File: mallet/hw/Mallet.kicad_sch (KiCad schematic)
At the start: 24 parts, among them J1 Conn_01x05, J2 Conn_01x03, J3 Conn_01x04, J4 Conn_01x04, U1 STM32G030F6Px, U2 AS5600L-ASOM, U3 DRV8313PWPR

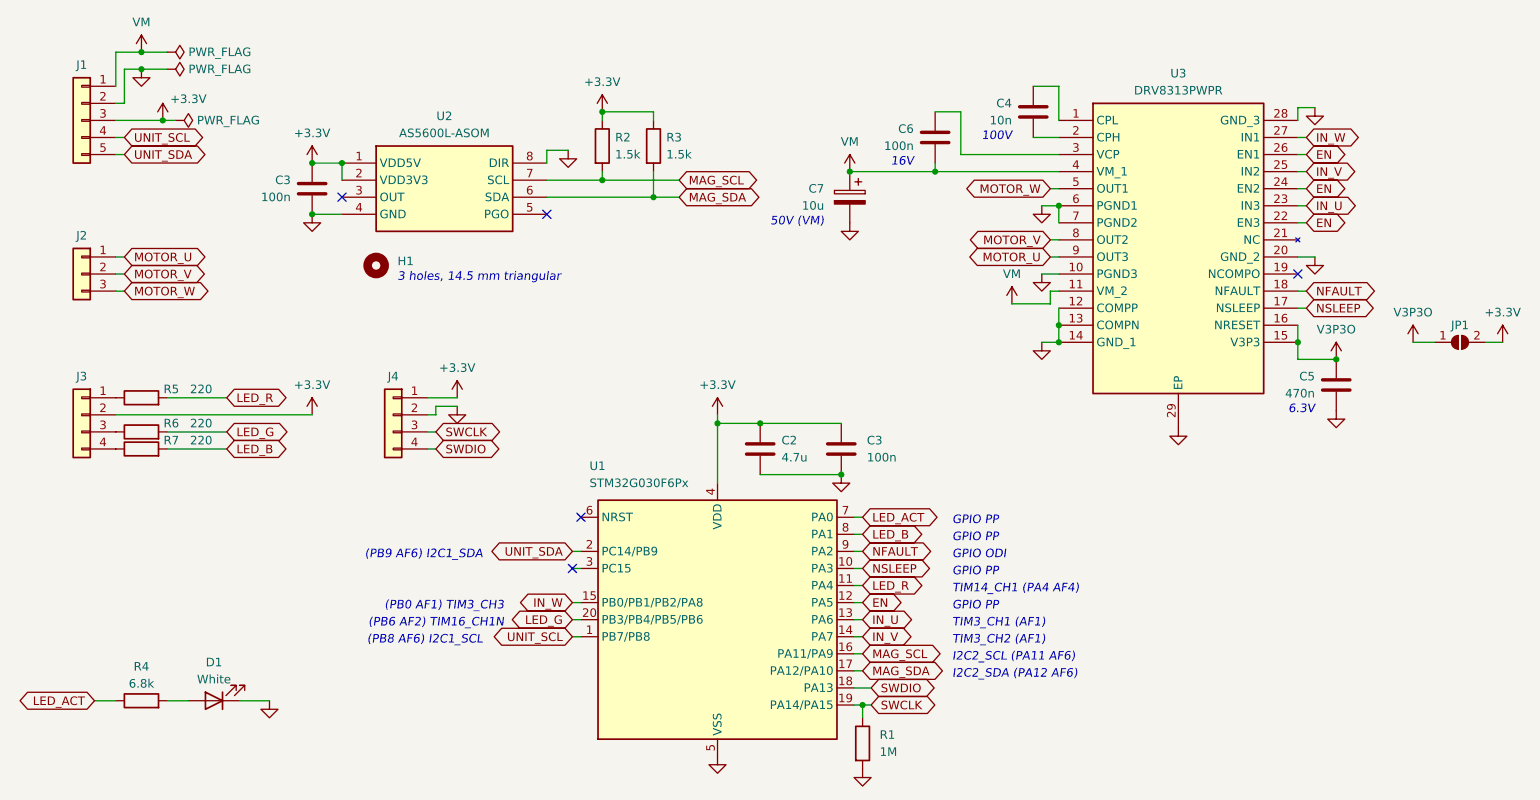
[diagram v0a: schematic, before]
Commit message: Finish mallet PCB
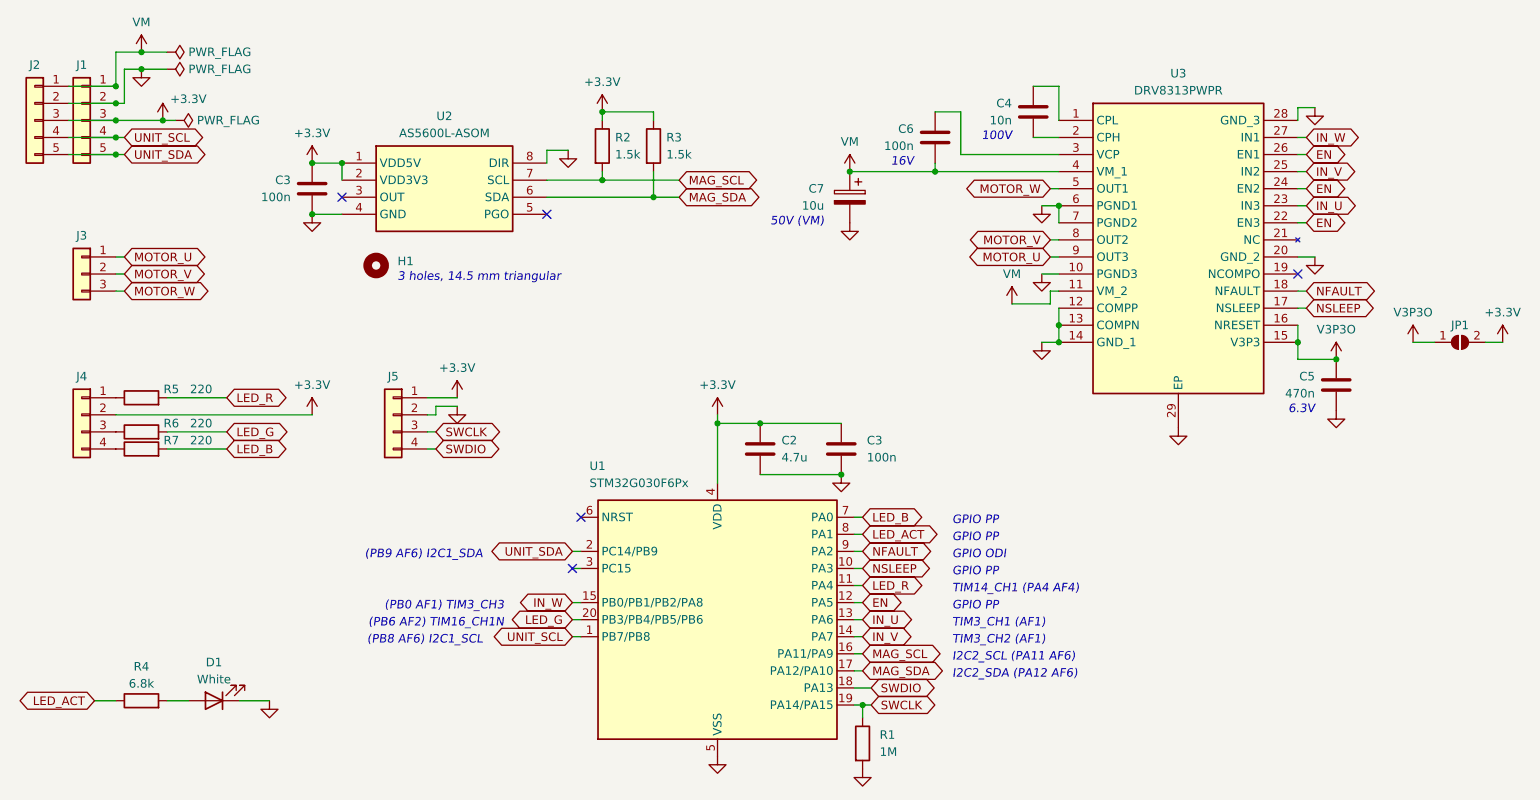
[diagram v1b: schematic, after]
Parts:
- added J2: Conn_01x05, Connector_PinHeader_2.00mm:PinHeader_1x05_P2.00mm_Vertical, symbol Connector_Generic:Conn_01x05
- C5: footprint Capacitor_SMD:C_0805_2012Metric -> Capacitor_SMD:C_0603_1608Metric
- J1: footprint Connector_PinHeader_2.00mm:PinHeader_1x04_P2.00mm_Vertical -> Connector_PinHeader_2.00mm:PinHeader_1x05_P2.00mm_Vertical
- renumbered J2 to J3, J3 to J4, J4 to J5
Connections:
- net +3.3V: now also J2.3 (Pin_3)
- net GND: now also J2.2 (Pin_2)
- net LED_ACT: now also U1.8 (PA1); no longer U1.7 (PA0)
- net LED_B: now also U1.7 (PA0); no longer U1.8 (PA1)
- net UNIT_SCL: now also J2.4 (Pin_4)
- net UNIT_SDA: now also J2.5 (Pin_5)
- net VM: now also J2.1 (Pin_1)
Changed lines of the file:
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@@
   (junction (at 156.845 38.735) (diameter 0) (color 0 0 0 0)
   )
+  (junction (at 34.925 26.035) (diameter 0) (color 0 0 0 0)
+  )
   (junction (at 175.26 61.595) (diameter 0) (color 0 0 0 0)
   )
@@
   (junction (at 114.935 42.545) (diameter 0) (color 0 0 0 0)
   )
+  (junction (at 34.925 31.115) (diameter 0) (color 0 0 0 0)
+  )
+  (junction (at 34.925 28.575) (diameter 0) (color 0 0 0 0)
+  )
   (junction (at 175.26 64.135) (diameter 0) (color 0 0 0 0)
   )
   (junction (at 38.735 20.955) (diameter 0) (color 0 0 0 0)
   )
+  (junction (at 34.925 33.655) (diameter 0) (color 0 0 0 0)
+  )
   (junction (at 68.58 37.465) (diameter 0) (color 0 0 0 0)
+  )
+  (junction (at 34.925 36.195) (diameter 0) (color 0 0 0 0)
   )
   (junction (at 124.46 76.2) (diameter 0) (color 0 0 0 0)
@@
     (stroke (width 0) (type default))
   )
+  (wire (pts (xy 27.94 33.655) (xy 34.925 33.655))
+    (stroke (width 0) (type default))
+  )
   (wire (pts (xy 146.05 92.71) (xy 144.78 92.71))
     (stroke (width 0) (type default))
@@
     (stroke (width 0) (type default))
   )
+  (wire (pts (xy 27.94 31.115) (xy 34.925 31.115))
+    (stroke (width 0) (type default))
+  )
   (wire (pts (xy 114.935 42.545) (xy 99.06 42.545))
     (stroke (width 0) (type default))
   )
+  (wire (pts (xy 27.94 28.575) (xy 34.925 28.575))
+    (stroke (width 0) (type default))
+  )
   (wire (pts (xy 227.965 64.135) (xy 231.14 64.135))
     (stroke (width 0) (type default))
@@
     (stroke (width 0) (type default))
   )
+  (wire (pts (xy 27.94 26.035) (xy 34.925 26.035))
+    (stroke (width 0) (type default))
+  )
   (wire (pts (xy 147.32 118.11) (xy 146.05 118.11))
     (stroke (width 0) (type default))
   )
   (wire (pts (xy 212.09 43.815) (xy 210.82 43.815))
+    (stroke (width 0) (type default))
+  )
+  (wire (pts (xy 27.94 36.195) (xy 34.925 36.195))
     (stroke (width 0) (type default))
   )
@@
     )
   )
-  (global_label "LED_B" (shape bidirectional) (at 146.05 92.71 0) (fields_autoplaced)
-    (effects (font (size 1.27 1.27)) (justify left))
-    (property "Intersheetrefs" "${INTERSHEET_REFS}" (at 155.8312 92.71 0)
+  (global_label "LED_ACT" (shape bidirectional) (at 146.05 92.71 0) (fields_autoplaced)
+    (effects (font (size 1.27 1.27)) (justify left))
+    (property "Intersheetrefs" "${INTERSHEET_REFS}" (at 157.8874 92.71 0)
       (effects (font (size 1.27 1.27)) (justify left) hide)
     )
@@
     )
   )
-  (global_label "LED_ACT" (shape bidirectional) (at 146.05 90.17 0) (fields_autoplaced)
-    (effects (font (size 1.27 1.27)) (justify left))
-    (property "Intersheetrefs" "${INTERSHEET_REFS}" (at 157.8874 90.17 0)
+  (global_label "LED_B" (shape bidirectional) (at 146.05 90.17 0) (fields_autoplaced)
+    (effects (font (size 1.27 1.27)) (justify left))
+    (property "Intersheetrefs" "${INTERSHEET_REFS}" (at 155.8312 90.17 0)
       (effects (font (size 1.27 1.27)) (justify left) hide)
     )
@@
       (effects (font (size 1.27 1.27)) (justify left))
     )
-    (property "Footprint" "Capacitor_SMD:C_0805_2012Metric" (at 215.5698 74.295 0)
+    (property "Footprint" "Capacitor_SMD:C_0603_1608Metric" (at 215.5698 74.295 0)
       (effects (font (size 1.27 1.27)) hide)
     )
@@
   (symbol (lib_id "Connector_Generic:Conn_01x03") (at 29.845 53.975 0) (mirror y) (unit 1)
     (in_bom yes) (on_board yes) (dnp no)
-    (property "Reference" "J2" (at 29.845 48.26 0)
+    (property "Reference" "J3" (at 29.845 48.26 0)
       (effects (font (size 1.27 1.27)))
     )
@@
       (project "Mallet"
         (path "/503c6fae-2261-4b98-b430-844cd1712448"
-          (reference "J2") (unit 1)
+          (reference "J3") (unit 1)
         )
       )
@@
   (symbol (lib_id "Connector_Generic:Conn_01x04") (at 76.2 74.93 0) (mirror y) (unit 1)
     (in_bom yes) (on_board yes) (dnp no)
-    (property "Reference" "J4" (at 76.2 69.215 0)
+    (property "Reference" "J5" (at 76.2 69.215 0)
       (effects (font (size 1.27 1.27)))
     )
@@
       (project "Mallet"
         (path "/503c6fae-2261-4b98-b430-844cd1712448"
-          (reference "J4") (unit 1)
+          (reference "J5") (unit 1)
         )
       )
@@
   (symbol (lib_id "Connector_Generic:Conn_01x04") (at 29.845 74.93 0) (mirror y) (unit 1)
     (in_bom yes) (on_board yes) (dnp no)
-    (property "Reference" "J3" (at 29.845 69.215 0)
+    (property "Reference" "J4" (at 29.845 69.215 0)
       (effects (font (size 1.27 1.27)))
     )
@@
       (project "Mallet"
         (path "/503c6fae-2261-4b98-b430-844cd1712448"
-          (reference "J3") (unit 1)
+          (reference "J4") (unit 1)
         )
       )
@@
       (effects (font (size 1.27 1.27)) hide)
     )
-    (property "Footprint" "Connector_PinHeader_2.00mm:PinHeader_1x04_P2.00mm_Vertical" (at 29.845 31.115 0)
+    (property "Footprint" "Connector_PinHeader_2.00mm:PinHeader_1x05_P2.00mm_Vertical" (at 29.845 31.115 0)
       (effects (font (size 1.27 1.27)) hide)
     )
@@
         )
       )
+    )
+  )
+  (symbol (lib_id "Connector_Generic:Conn_01x05") (at 22.86 31.115 0) (mirror y) (unit 1)
+    (in_bom yes) (on_board yes) (dnp no)
+    (property "Reference" "J2" (at 22.86 22.86 0)
+      (effects (font (size 1.27 1.27)))
+    )
+    (property "Value" "Conn_01x05" (at 22.86 41.275 0)
+      (effects (font (size 1.27 1.27)) hide)
+    )
+    (property "Footprint" "Connector_PinHeader_2.00mm:PinHeader_1x05_P2.00mm_Vertical" (at 22.86 31.115 0)
+      (effects (font (size 1.27 1.27)) hide)
+    )
+    (property "Datasheet" "~" (at 22.86 31.115 0)
+      (effects (font (size 1.27 1.27)) hide)
+    )
+    (pin "2")
+    (pin "5")
+    (pin "4")
+    (pin "1")
+    (pin "3")
+    (instances
+      (project "Mallet"
+        (path "/503c6fae-2261-4b98-b430-844cd1712448"
+          (reference "J2") (unit 1)
+        )
+      )
